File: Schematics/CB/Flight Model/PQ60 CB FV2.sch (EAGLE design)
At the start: 29 parts, among them U1 ATMEGA328P-AU, U2 LSM9DS0, U3 LTC2990IMSPBF

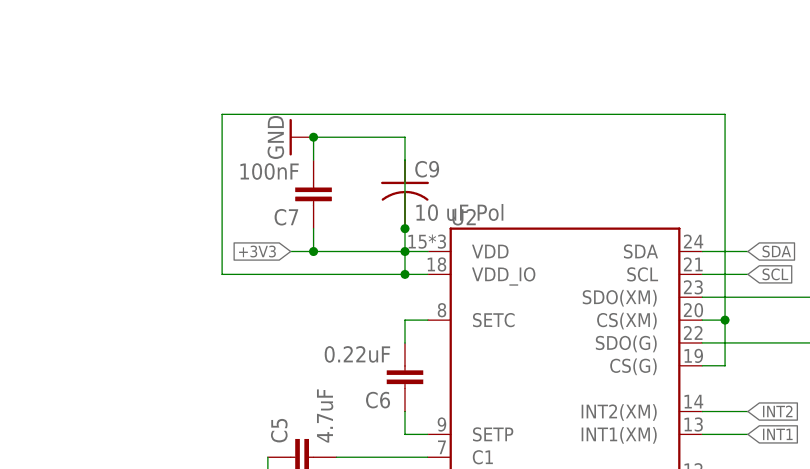
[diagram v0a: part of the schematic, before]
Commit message: m
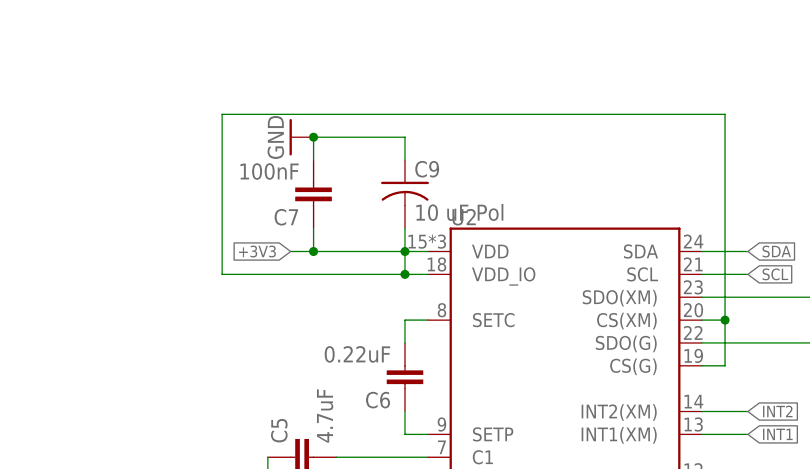
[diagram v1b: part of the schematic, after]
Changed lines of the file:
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@@
 <junction x="58.42" y="391.16"/>
 <pinref part="C9" gate="G$1" pin="1"/>
-<wire x1="68.58" y1="388.62" x2="68.58" y2="391.16" width="0.1524" layer="91"/>
+<wire x1="68.58" y1="391.16" x2="68.58" y2="388.62" width="0.1524" layer="91"/>
 </segment>
 <segment>
@@
 <wire x1="58.42" y1="381" x2="58.42" y2="378.46" width="0.1524" layer="91"/>
 <junction x="58.42" y="378.46"/>
-<wire x1="68.58" y1="388.62" x2="68.58" y2="381" width="0.1524" layer="91"/>
 <junction x="68.58" y="378.46"/>
 <pinref part="U2" gate="G$1" pin="VDD_IO"/>
@@
 <junction x="104.14" y="370.84"/>
 <pinref part="C9" gate="G$1" pin="2"/>
-<junction x="68.58" y="381"/>
 </segment>
 <segment>
